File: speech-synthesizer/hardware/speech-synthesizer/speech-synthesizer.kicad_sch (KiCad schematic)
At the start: 33 parts, among them J1 AudioJack3, Q1 BS250, U1 TMS5220C, U2 ATF22V10C, U3 74HCT245, U4 74HCT374, U5 74HCT374, U6 74HCT74, U7 74HCT688, U8 74HCT688

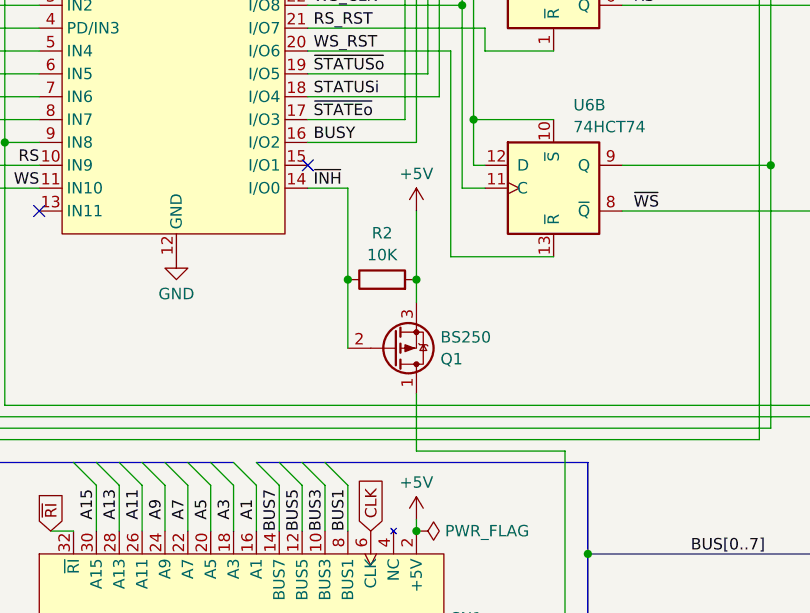
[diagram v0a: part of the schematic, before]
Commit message: improved backplane
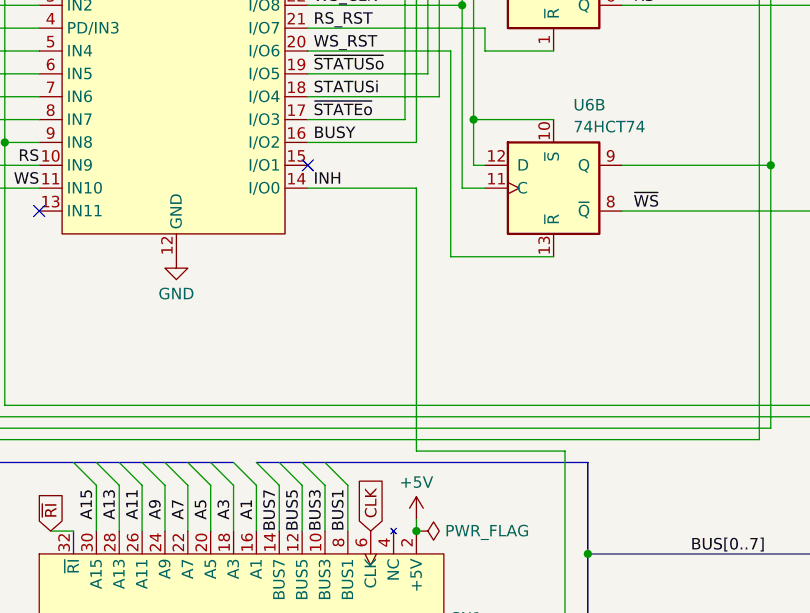
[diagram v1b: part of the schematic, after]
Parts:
- removed Q1: BS250, Package_TO_SOT_THT:TO-92_Inline, symbol Transistor_FET:BS250
- removed R2: 10K, Resistor_THT:R_Axial_DIN0207_L6.3mm_D2.5mm_P10.16mm_Horizontal, symbol Device:R
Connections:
- net ~{INH} is gone; now on net INH: U2.14 (I/O0)
